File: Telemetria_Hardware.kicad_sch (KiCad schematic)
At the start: 16 parts, among them M100A1 1715734

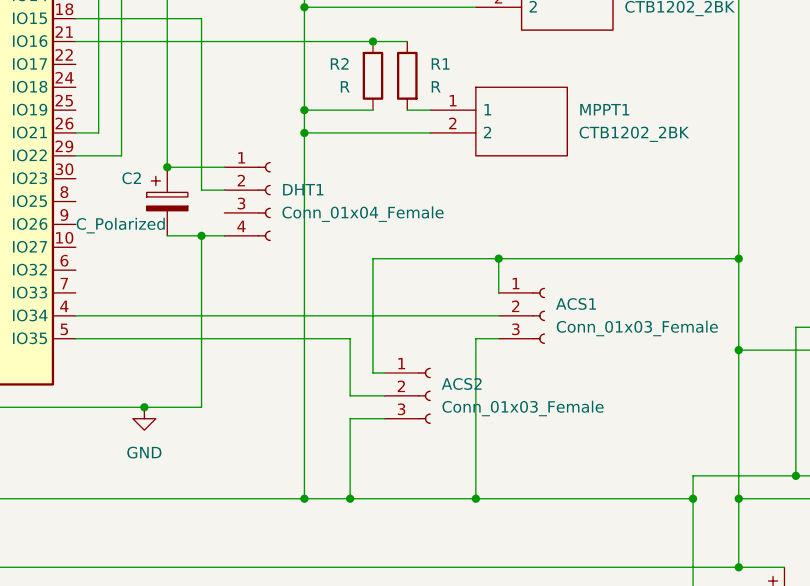
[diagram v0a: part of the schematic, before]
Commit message: ads adicionado
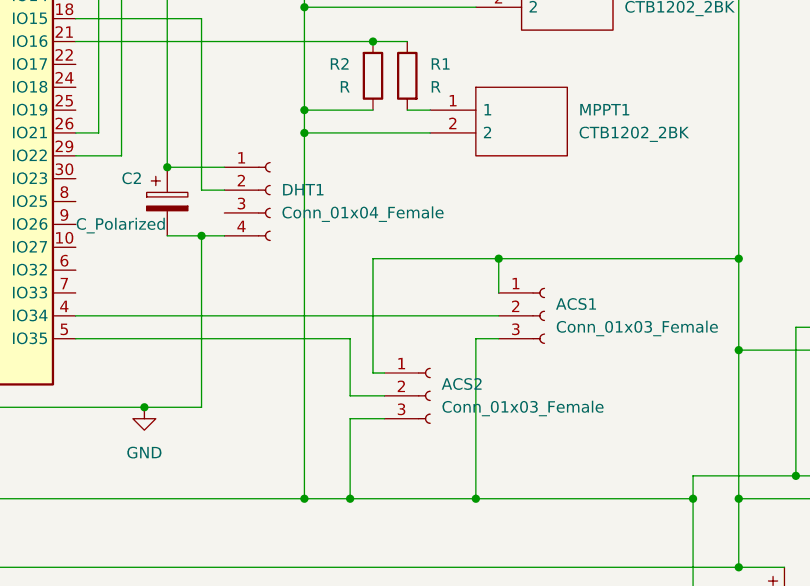
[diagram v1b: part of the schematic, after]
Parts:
- ESP32: footprint esp32_devkit_v1_doit:esp32_devkit_v1_doit -> ESP32-DOIT-DEVKIT:ESP32-DOIT-DEVKIT

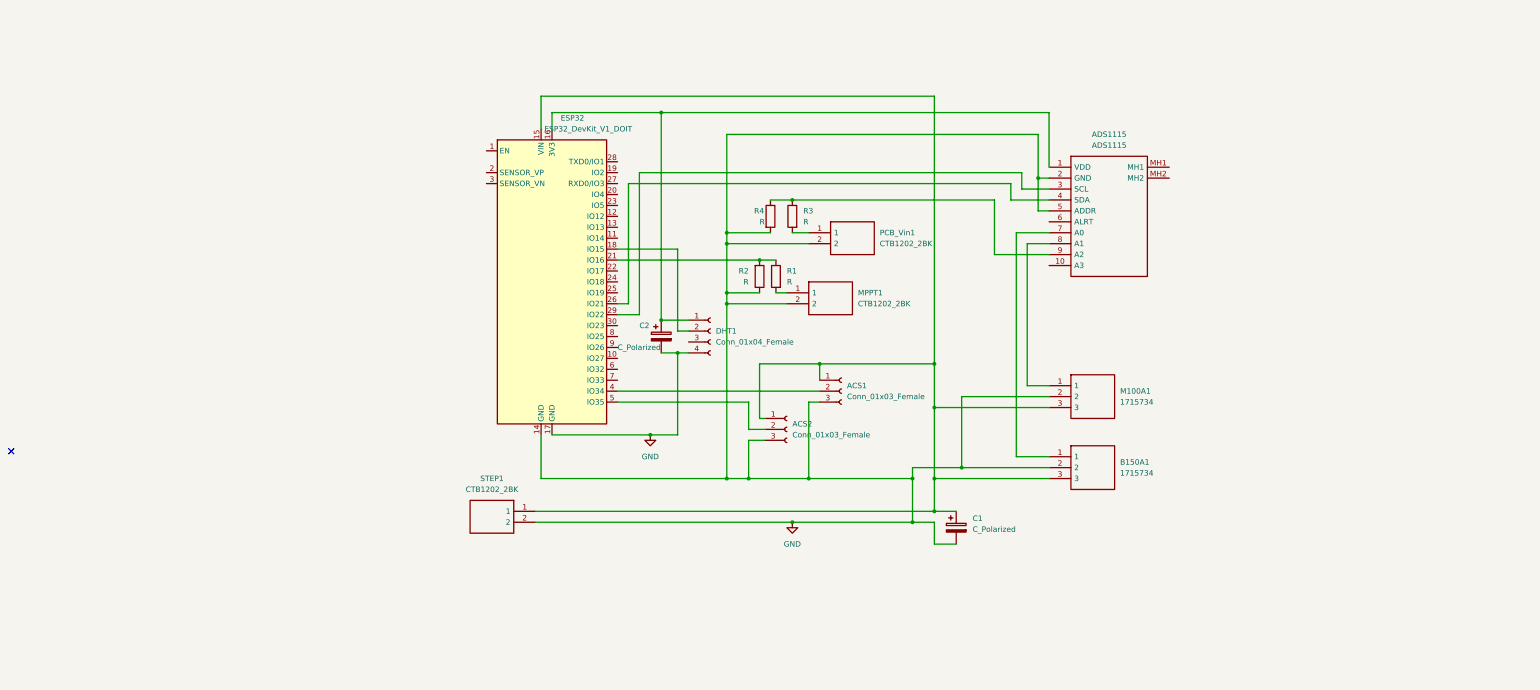
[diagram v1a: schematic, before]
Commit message: placa teste
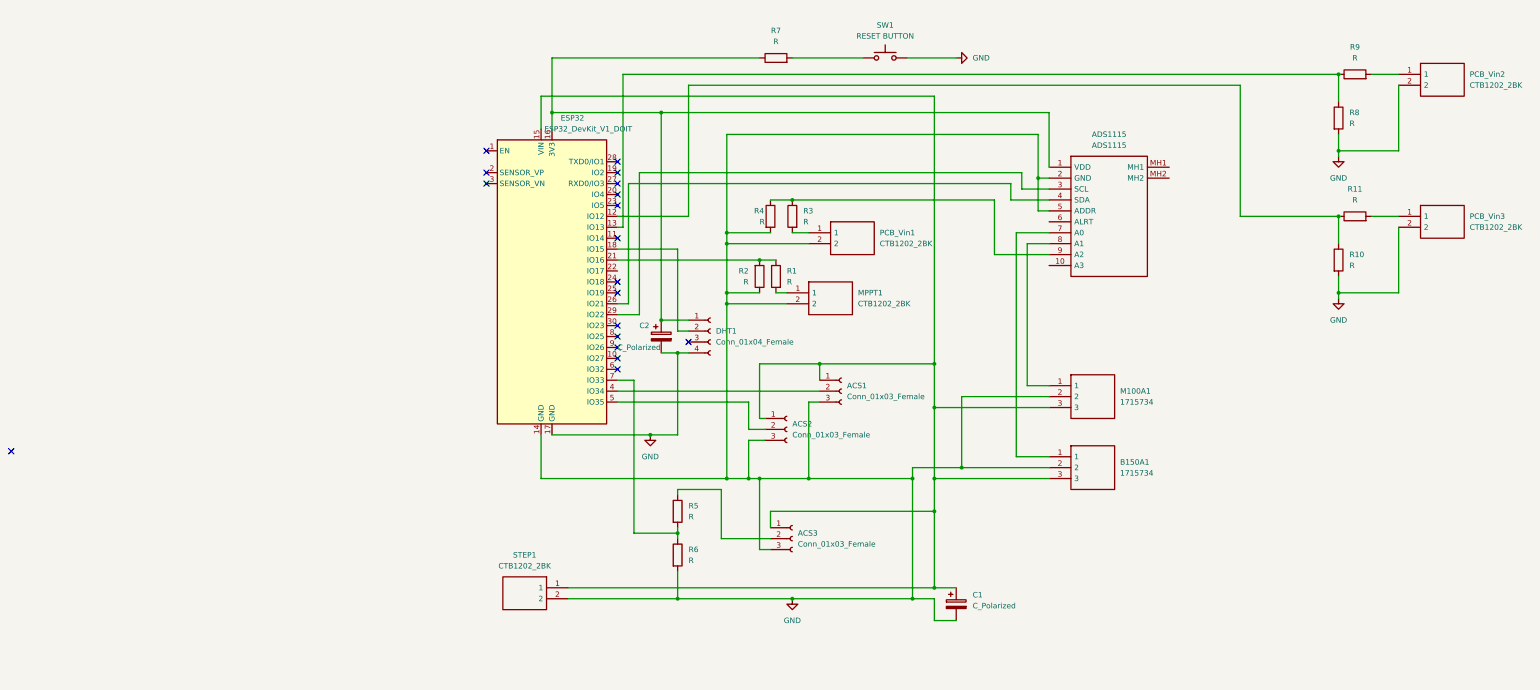
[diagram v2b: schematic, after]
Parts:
- added ACS3: Conn_01x03_Female, Connector_PinSocket_2.54mm:PinSocket_1x03_P2.54mm_Vertical, symbol Connector:Conn_01x03_Female
- added PCB_Vin2, PCB_Vin3: CTB1202_2BK, TerminalBlock:TerminalBlock_bornier-2_P5.08mm, symbol KRE_Terminal_2Way_5.08mm:CTB1202_2BK
- added R10, R11, R5, R6, R7, R8, R9: R, Resistor_THT:R_Axial_DIN0207_L6.3mm_D2.5mm_P10.16mm_Horizontal, symbol Device:R
- added SW1: RESET BUTTON, symbol Switch:SW_MEC_5G
- B150A1, M100A1: footprint Terminal_Block_PCB_3Way:Connector_KRE_3W_5,08mm -> TerminalBlock:TerminalBlock_bornier-3_P5.08mm
- MPPT1, PCB_Vin1, STEP1: footprint Terminal_Block_PCB_2Way:KRE_Terminal_2Way_5.08mm -> TerminalBlock:TerminalBlock_bornier-2_P5.08mm
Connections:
- net GND: now also ACS3.3 (Pin_3), PCB_Vin2.2, PCB_Vin3.2, R10.2, R6.2, R8.2, SW1.3 (B), SW1.4 (B)
- net at ESP32.12 (IO12): now also R10.1, R11.1
- net at ESP32.13 (IO13): now also R8.1, R9.1
- net at ACS1.1 (Pin_1), ACS2.1 (Pin_1), B150A1.3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: now also ACS3.1 (Pin_1)
- net at ADS1115.1 (VDD), C2.1, DHT1.1 (Pin_1)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: now also R7.1
- net at ESP32.7 (IO33): now also R5.2, R6.1
- new net: PCB_Vin2.1, R9.2
- new net: PCB_Vin3.1, R11.2
- new net: R7.2, SW1.1 (A), SW1.2 (A)
- new net: ACS3.2 (Pin_2), R5.1
- no-connect marks 1 -> 18
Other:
- moved on the sheet: C1, STEP1

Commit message: teste 2
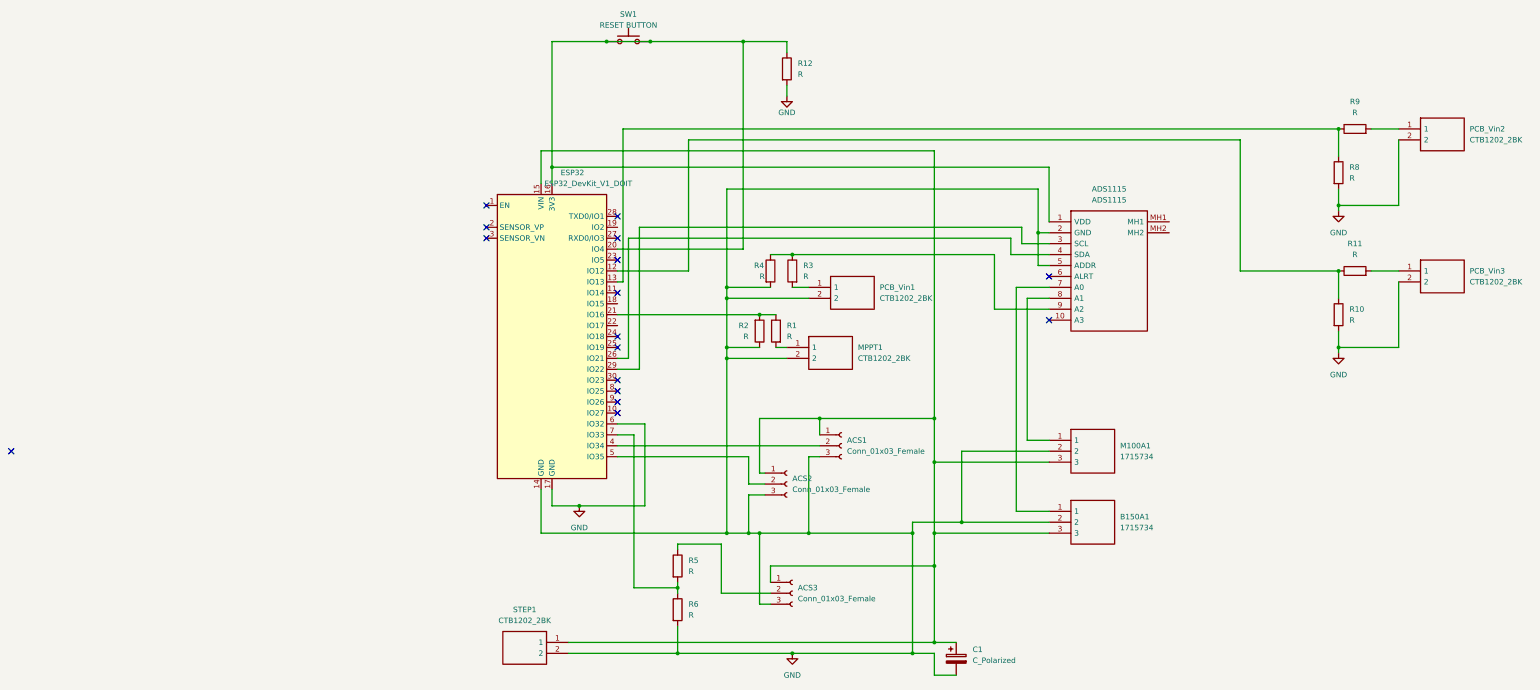
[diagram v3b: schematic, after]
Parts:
- removed C2: C_Polarized, Capacitor_THT:C_Radial_D6.3mm_H11.0mm_P2.50mm, symbol Device:C_Polarized
- removed DHT1: Conn_01x04_Female, Connector_PinSocket_2.54mm:PinSocket_1x04_P2.54mm_Vertical, symbol Connector:Conn_01x04_Female
- removed R7: R, Resistor_THT:R_Axial_DIN0207_L6.3mm_D2.5mm_P10.16mm_Horizontal, symbol Device:R
- added R12: R, Resistor_THT:R_Axial_DIN0207_L6.3mm_D2.5mm_P10.16mm_Horizontal, symbol Device:R
- ESP32: footprint ESP32-DOIT-DEVKIT:ESP32-DOIT-DEVKIT -> ESP32:esp32_devkit_v1_doit
- SW1: footprint (none) -> BUTT:BUTT
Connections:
- net GND: now also ESP32.6 (IO32), R12.2; no longer SW1.3 (B), SW1.4 (B)
- net at ADS1115.1 (VDD), ESP32.16 (3V3): now also ESP32.20 (IO4), SW1.1 (A), SW1.2 (A), SW1.3 (B), SW1.4 (B), R12.1
- no-connect marks 18 -> 16
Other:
- moved on the sheet: ACS1, ACS2, ACS3, ADS1115, B150A1, C1, ESP32, M100A1, MPPT1, PCB_Vin1, PCB_Vin2, PCB_Vin3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
